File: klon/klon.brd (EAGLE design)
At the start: 160 x 100 mm, 14 parts, among them IC1 MAX1044

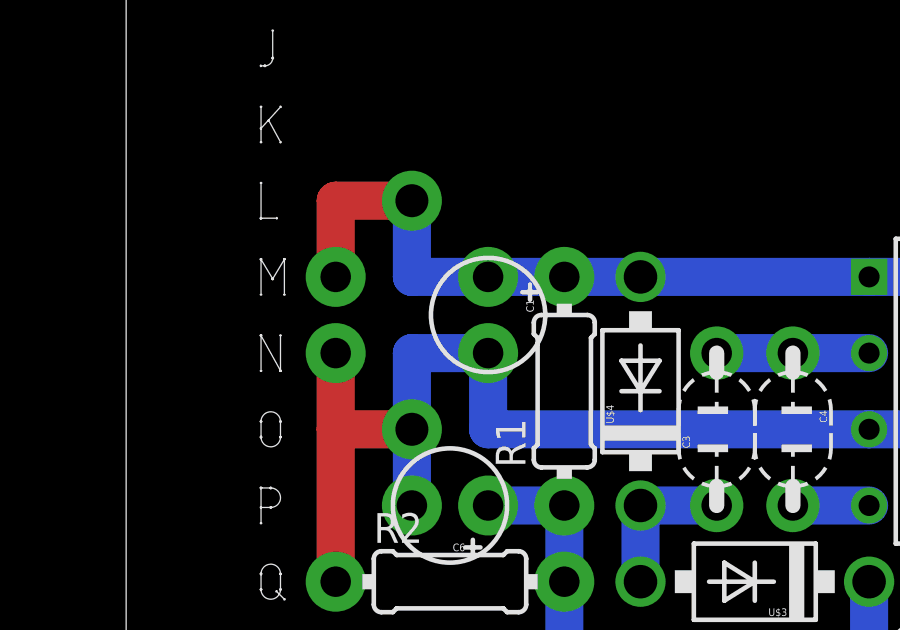
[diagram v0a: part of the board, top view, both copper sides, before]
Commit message: klon tweaks
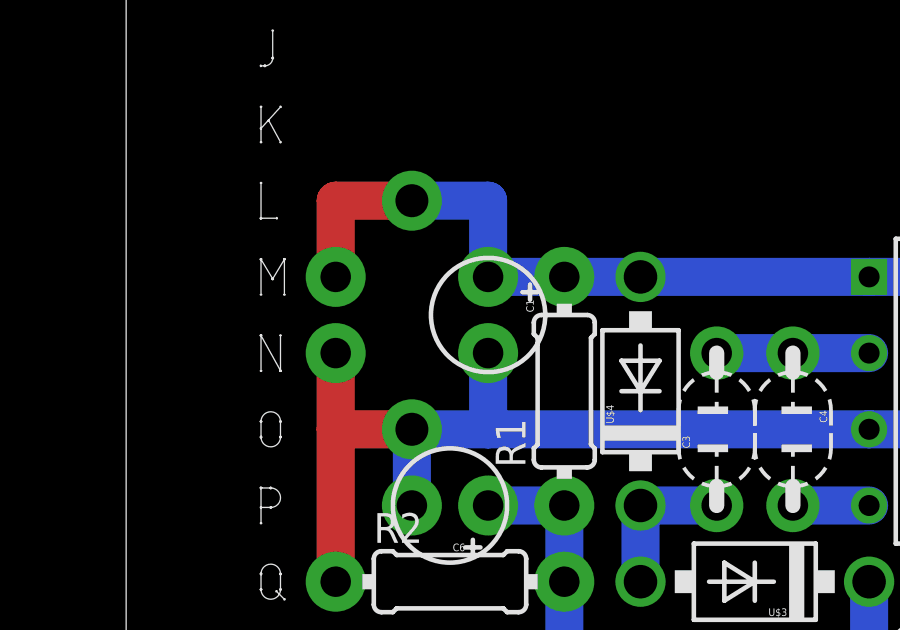
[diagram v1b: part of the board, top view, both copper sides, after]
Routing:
- net GND: track 45.7 -> 43.2 mm
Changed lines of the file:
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@@
 <wire x1="15.24" y1="48.26" x2="15.24" y2="50.8" width="1.27" layer="1"/>
 <wire x1="15.24" y1="50.8" x2="17.78" y2="50.8" width="1.27" layer="1"/>
-<wire x1="20.32" y1="48.26" x2="17.78" y2="48.26" width="1.27" layer="16"/>
-<wire x1="17.78" y1="48.26" x2="17.78" y2="50.8" width="1.27" layer="16"/>
 <wire x1="40.64" y1="48.26" x2="33.02" y2="48.26" width="1.27" layer="16"/>
 <wire x1="25.4" y1="48.26" x2="22.86" y2="48.26" width="1.27" layer="16"/>
 <wire x1="20.32" y1="48.26" x2="22.86" y2="48.26" width="1.27" layer="16"/>
 <wire x1="25.4" y1="48.26" x2="33.02" y2="48.26" width="1.27" layer="16"/>
+<wire x1="17.78" y1="50.8" x2="20.32" y2="50.8" width="1.27" layer="16"/>
+<wire x1="20.32" y1="50.8" x2="20.32" y2="48.26" width="1.27" layer="16"/>
 </signal>
 <signal name="+16.2V">
@@
 <wire x1="15.24" y1="45.72" x2="15.24" y2="43.18" width="1.27" layer="1"/>
 <wire x1="15.24" y1="43.18" x2="17.78" y2="43.18" width="1.27" layer="1"/>
-<wire x1="20.32" y1="45.72" x2="17.78" y2="45.72" width="1.27" layer="16"/>
-<wire x1="17.78" y1="45.72" x2="17.78" y2="43.18" width="1.27" layer="16"/>
 <wire x1="15.24" y1="38.1" x2="15.24" y2="43.18" width="1.27" layer="1"/>
 <wire x1="17.78" y1="40.64" x2="17.78" y2="43.18" width="1.27" layer="16"/>
@@
 <wire x1="38.1" y1="35.56" x2="35.56" y2="35.56" width="1.27" layer="16"/>
 <wire x1="35.56" y1="35.56" x2="35.56" y2="38.1" width="1.27" layer="16"/>
+<wire x1="17.78" y1="43.18" x2="20.32" y2="43.18" width="1.27" layer="16"/>
 </signal>
 <signal name="N$2">
